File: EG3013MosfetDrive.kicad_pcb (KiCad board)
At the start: 2 copper layers, 38 x 30.5 mm, 36 parts, among them J1 Conn_02x03_Odd_Even, Q1 QM6006D, Q2 QM6006D, Q3 QM6006D, Q4 QM6006D, U1 EG3013, U2 EG3013

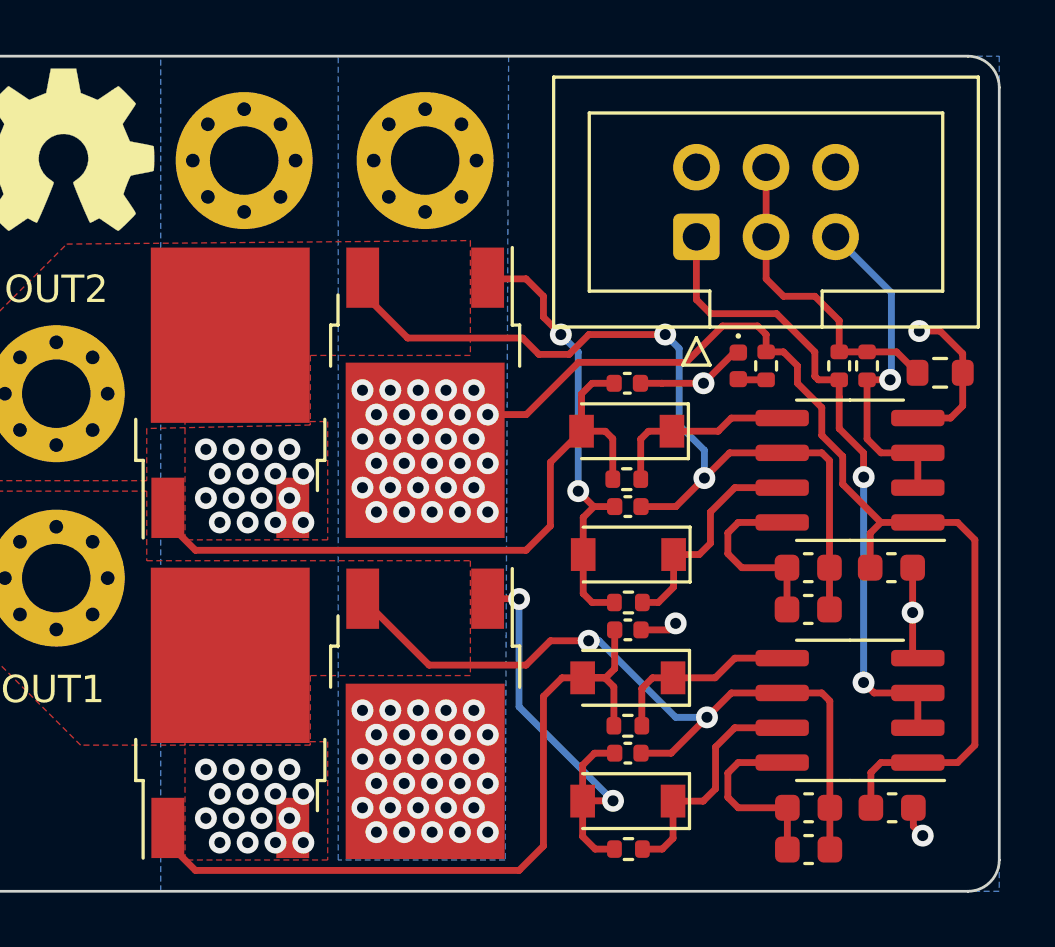
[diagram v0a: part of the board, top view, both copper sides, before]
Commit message: fix some net
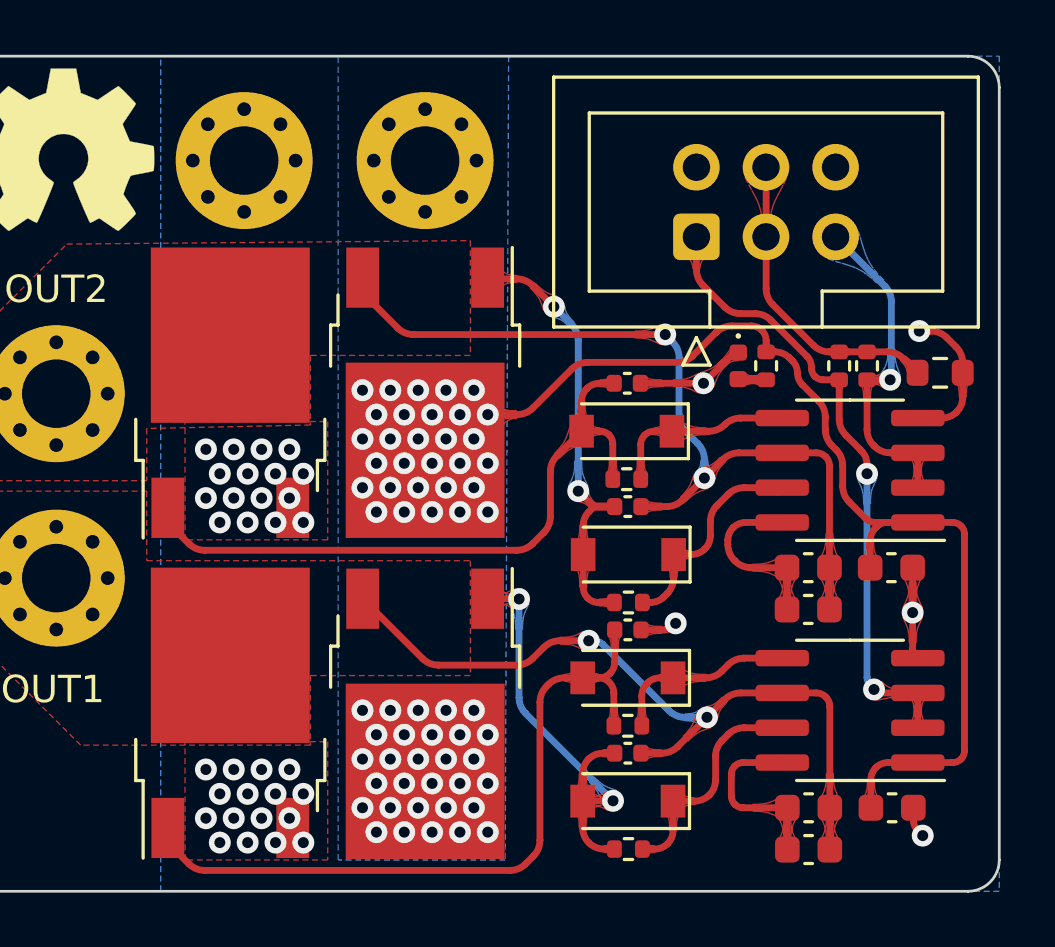
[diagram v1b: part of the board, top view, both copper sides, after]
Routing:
- net IN1: track 24.1 -> 22.7 mm
- net OUT2: track 31.9 -> 31.0 mm
- net +12V: track 40.0 -> 39.4 mm

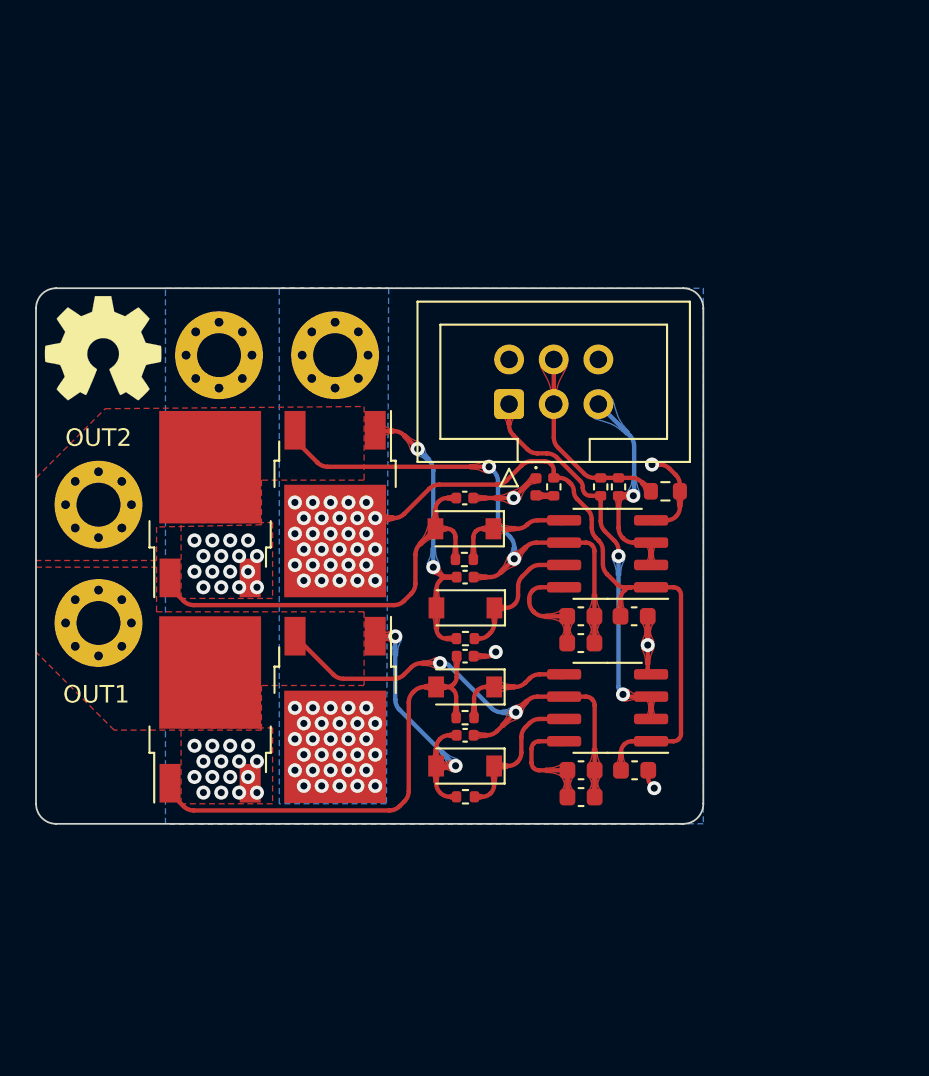
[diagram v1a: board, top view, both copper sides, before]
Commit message: model D Vesion
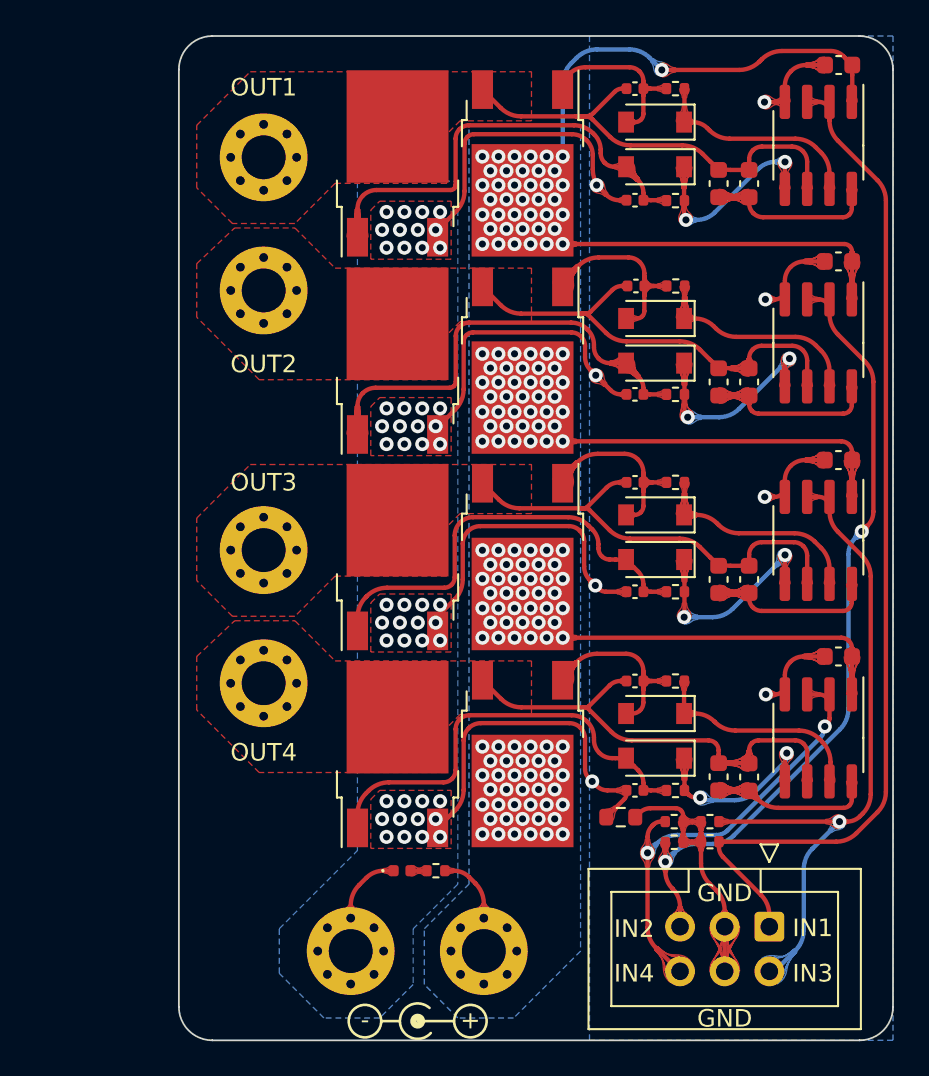
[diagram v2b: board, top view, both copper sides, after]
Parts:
- removed the REF** at (107.4, 85.1)
- added C11: 100nF, Capacitor_SMD:C_0603_1608Metric, F.Cu at (149.3, 80.1)
- added C12: 100nF, Capacitor_SMD:C_0603_1608Metric, F.Cu at (149.3, 102.6)
- added C13: 10nF, Capacitor_SMD:C_0402_1005Metric, F.Cu at (137.8, 81.5)
- added C14: 10nF, Capacitor_SMD:C_0402_1005Metric, F.Cu at (137.7, 87.7)
- added C15: 10nF, Capacitor_SMD:C_0402_1005Metric, F.Cu at (137.7, 104.0)
- added C16: 10nF, Capacitor_SMD:C_0402_1005Metric, F.Cu at (137.7, 110.2)
- added C17: 22uF, Capacitor_SMD:C_0603_1608Metric, F.Cu at (144.2, 87.0)
- added C18: 22uF, Capacitor_SMD:C_0603_1608Metric, F.Cu at (142.5, 109.5)
- added C19: 22uF, Capacitor_SMD:C_0603_1608Metric, F.Cu at (142.5, 87.0)
- added C20: 22uF, Capacitor_SMD:C_0603_1608Metric, F.Cu at (144.2, 109.5)
- added D6: 1N4148, Diode_SMD:D_SOD-123, F.Cu at (138.9, 83.4)
- added D7: 1N4148, Diode_SMD:D_SOD-123, F.Cu at (138.9, 85.9)
- added D8: 1N4148, Diode_SMD:D_SOD-123, F.Cu at (138.9, 105.9)
- added D9: 1N4148, Diode_SMD:D_SOD-123, F.Cu at (138.9, 108.4)
- added H5: Pad, MountingHole:MountingHole_2.5mm_Pad_Via, F.Cu at (116.6, 81.8)
- added H6: Pad, MountingHole:MountingHole_2.5mm_Pad_Via, F.Cu at (116.6, 104.1)
- added Q5: QM6006D, Package_TO_SOT_SMD:TO-252-2, F.Cu at (131.3, 85.8)
- added Q6: QM6006D, Package_TO_SOT_SMD:TO-252-2, F.Cu at (124.2, 85.8)
- added Q7: QM6006D, Package_TO_SOT_SMD:TO-252-2, F.Cu at (131.3, 108.2)
- added Q8: QM6006D, Package_TO_SOT_SMD:TO-252-2, F.Cu at (124.2, 108.2)
- added R10: 1k, Resistor_SMD:R_0402_1005Metric, F.Cu at (139.9, 112.0)
- added R11: 22R, Resistor_SMD:R_0402_1005Metric, F.Cu at (140.0, 81.5)
- added R12: 22R, Resistor_SMD:R_0402_1005Metric, F.Cu at (140.0, 87.7)
- added R13: 22R, Resistor_SMD:R_0402_1005Metric, F.Cu at (140.0, 104.0)
- added R14: 22R, Resistor_SMD:R_0402_1005Metric, F.Cu at (140.0, 110.2)
- added R9: 1k, Resistor_SMD:R_0402_1005Metric, F.Cu at (142.0, 112.0)
- added REF**: Symbol_Barrel_Polarity, Symbol:Symbol_Barrel_Polarity, F.Cu at (125.3, 123.3)
- added REF**: Symbol_Barrel_Polarity, Symbol:Symbol_Barrel_Polarity, B.Cu at (125.3, 123.4)
- added REF**: OSHW-Symbol_8.9x8mm_SilkScreen, Symbol:OSHW-Symbol_8.9x8mm_SilkScreen, B.Cu at (143.4, 73.8)
- added U3: EG3013, Package_SO:SOIC-8_3.9x4.9mm_P1.27mm, F.Cu at (148.1, 84.8)
- added U4: EG3013, Package_SO:SOIC-8_3.9x4.9mm_P1.27mm, F.Cu at (148.1, 107.2)
- C1, C2: value 10nF -> 100nF; footprint Capacitor_SMD:C_0402_1005Metric -> Capacitor_SMD:C_0603_1608Metric
- C10, C9: value 100nF -> 22uF
- C5, C6: value 22uF -> 10nF; footprint Capacitor_SMD:C_0603_1608Metric -> Capacitor_SMD:C_0402_1005Metric
- D1: value 1N4148 -> LED_Small; footprint Diode_SMD:D_SOD-123 -> LED_SMD:LED_0402_1005Metric
- D5: value LED_Small -> 1N4148; footprint LED_SMD:LED_0402_1005Metric -> Diode_SMD:D_SOD-123
- R1: value 22R -> 0R; footprint Resistor_SMD:R_0402_1005Metric -> Resistor_SMD:R_0603_1608Metric
- R2: value 22R -> 4.7k
- R5: value 4.7k -> 22R
- R6: value 0R -> 22R; footprint Resistor_SMD:R_0603_1608Metric -> Resistor_SMD:R_0402_1005Metric
- moved C2 39.8 mm to (149.3, 69.0)
- moved C7 34.7 mm to (144.2, 75.7), turned to 90 degrees
- moved H1 34.7 mm to (121.5, 119.4), turned to -90 degrees
- moved U1 34.2 mm to (148.1, 73.5), turned to -90 degrees
- moved D2 33.9 mm to (138.9, 72.2)
- moved H4 33.6 mm to (129.1, 119.4), turned to -90 degrees
- moved R3 33.5 mm to (140.0, 70.3)
- moved J1 33.2 mm to (145.4, 118.0), turned to -90 degrees
- moved Q1 32.9 mm to (131.3, 74.6)
- moved Q2 32.8 mm to (124.2, 74.6)
- moved C3 29.4 mm to (137.7, 70.3), turned to 0 degrees
- moved D3 27.3 mm to (138.9, 74.7)
- moved C1 26.4 mm to (149.3, 91.4)
- moved C9 25.1 mm to (142.5, 75.7), turned to 90 degrees
- moved R4 23.7 mm to (140.0, 76.7)
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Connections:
- C1 pad 1: OUT1 -> +12V
- C1 pad 2: Net-(C1-Pad2) -> GNDPWR
- C10 pad 1: +12V -> Net-(C10-Pad1)
- C10 pad 2: GNDPWR -> OUT3
- C2 pad 1: GNDPWR -> +12V
- C2 pad 2: Net-(C2-Pad2) -> GNDPWR
- C3 pad 1: OUT2 -> OUT1
- C5 pad 1: Net-(C5-Pad1) -> OUT3
- C5 pad 2: OUT1 -> Net-(C5-Pad2)
- C6 pad 1: Net-(C6-Pad1) -> GNDPWR
- C6 pad 2: OUT2 -> Net-(C6-Pad2)
- C7 pad 1: Net-(C5-Pad1) -> Net-(C7-Pad1)
- C8 pad 1: Net-(C6-Pad1) -> Net-(C10-Pad1)
- C8 pad 2: OUT2 -> OUT3
- C9 pad 1: +12V -> Net-(C7-Pad1)
- C9 pad 2: GNDPWR -> OUT1
- D1 pad 1: Net-(D1-Pad1) -> GNDPWR
- D1 pad 2: Net-(C1-Pad2) -> Net-(D1-Pad2)
- D2 pad 2: Net-(C2-Pad2) -> Net-(C3-Pad2)
- D3 pad 2: Net-(C3-Pad2) -> Net-(C4-Pad2)
- D4 pad 2: Net-(C4-Pad2) -> Net-(C5-Pad2)
- D5 pad 1: GNDPWR -> Net-(D5-Pad1)
- D5 pad 2: Net-(D5-Pad2) -> Net-(C6-Pad2)
- H2 pad 1: +12V -> OUT1
- H3 pad 1: OUT1 -> OUT3
- H4 pad 1: OUT2 -> +12V
- J1 pad 2: unconnected-(J1-Pad2) -> IN3
- J1 pad 6: unconnected-(J1-Pad6) -> IN4
- Q1 pad 1: Net-(C1-Pad2) -> Net-(C3-Pad2)
- Q2 pad 1: Net-(C2-Pad2) -> Net-(C4-Pad2)
- Q3 pad 1: Net-(C3-Pad2) -> Net-(C5-Pad2)
- Q3 pad 3: OUT2 -> OUT3
- Q4 pad 1: Net-(C4-Pad2) -> Net-(C6-Pad2)
- Q4 pad 2: OUT2 -> OUT3
- R1 pad 1: Net-(C1-Pad2) -> GNDPWR
- R1 pad 2: Net-(D1-Pad1) -> GND
- R2 pad 1: Net-(C2-Pad2) -> +12V
- R2 pad 2: Net-(D2-Pad1) -> Net-(D1-Pad2)
- R3 pad 2: Net-(D3-Pad1) -> Net-(D2-Pad1)
- R4 pad 2: Net-(D4-Pad1) -> Net-(D3-Pad1)
- R5 pad 1: +12V -> Net-(C5-Pad2)
- R5 pad 2: Net-(D5-Pad2) -> Net-(D4-Pad1)
- R6 pad 1: GNDPWR -> Net-(C6-Pad2)
- R6 pad 2: GND -> Net-(D5-Pad1)
- U1 pad 5: Net-(D2-Pad1) -> Net-(D3-Pad1)
- U1 pad 7: Net-(D1-Pad1) -> Net-(D2-Pad1)
- U1 pad 8: Net-(C5-Pad1) -> Net-(C7-Pad1)
- U2 pad 2: IN2 -> IN3
- U2 pad 3: IN2 -> IN3
- U2 pad 5: Net-(D4-Pad1) -> Net-(D5-Pad1)
- U2 pad 6: OUT2 -> OUT3
- U2 pad 7: Net-(D3-Pad1) -> Net-(D4-Pad1)
- U2 pad 8: Net-(C6-Pad1) -> Net-(C10-Pad1)
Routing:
- net GNDPWR: track 15.4 -> 101.8 mm, vias 37 -> 56
- net +12V: track 39.4 -> 88.9 mm, vias 60 -> 157
- net IN3: track 0.00 -> 38.4 mm, vias 0 -> 1
- net IN1: track 22.7 -> 58.1 mm, vias 2 -> 0
- net IN2: track 12.2 -> 44.8 mm, vias 1 -> 2
- net Net-(C2-Pad2): track 28.0 -> 0.00 mm
- net OUT4: track 0.00 -> 26.6 mm
- net OUT3: track 0.00 -> 26.1 mm
- net IN4: track 0.00 -> 25.9 mm, vias 0 -> 2
- net Net-(C14-Pad2): track 0.00 -> 25.3 mm
- net Net-(C6-Pad2): track 0.00 -> 24.9 mm
- net Net-(C16-Pad2): track 0.00 -> 24.9 mm
- net Net-(C1-Pad2): track 16.2 -> 0.00 mm, vias 2 -> 0
- net Net-(D8-Pad1): track 0.00 -> 13.3 mm
- net Net-(D6-Pad1): track 0.00 -> 12.3 mm
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- added copper zone on F.Cu, net OUT3
- added copper zone on F.Cu, net OUT4
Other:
- board size 38 x 30.5 mm -> 40.6 x 57.1 mm
- board text added: "+"
- board text added: "-"
- board text added: "IN3"
- board text added: "IN4"
- board text added: "OUT3"
- board text added: "OUT4"
- board text removed: "Designed by zenchrer with Kicad"
- board text removed: "NC"
